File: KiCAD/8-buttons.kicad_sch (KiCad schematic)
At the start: 3 parts, among them U1 74HC165, U2 TLC5916

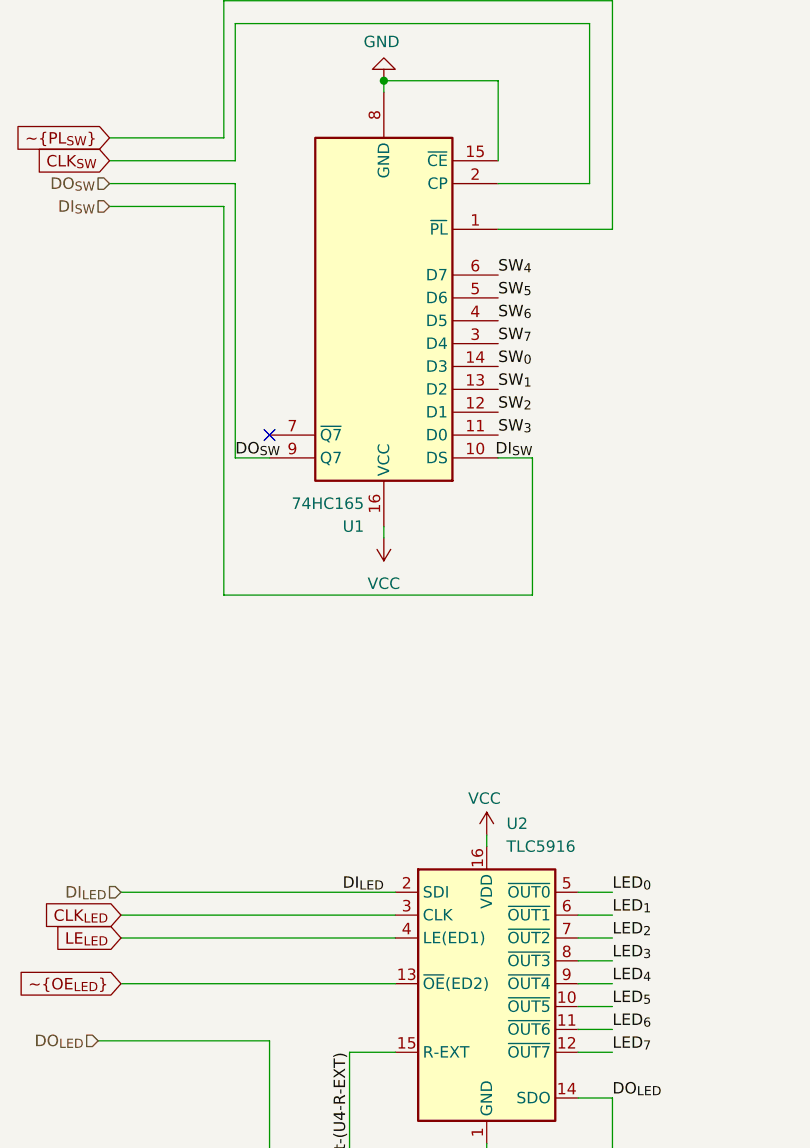
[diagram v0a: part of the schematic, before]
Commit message: Revert "3 rows of 16 buttons; SMT"
This reverts commit c08e4dc0c350e57a2ca7329c2459be699e742724.
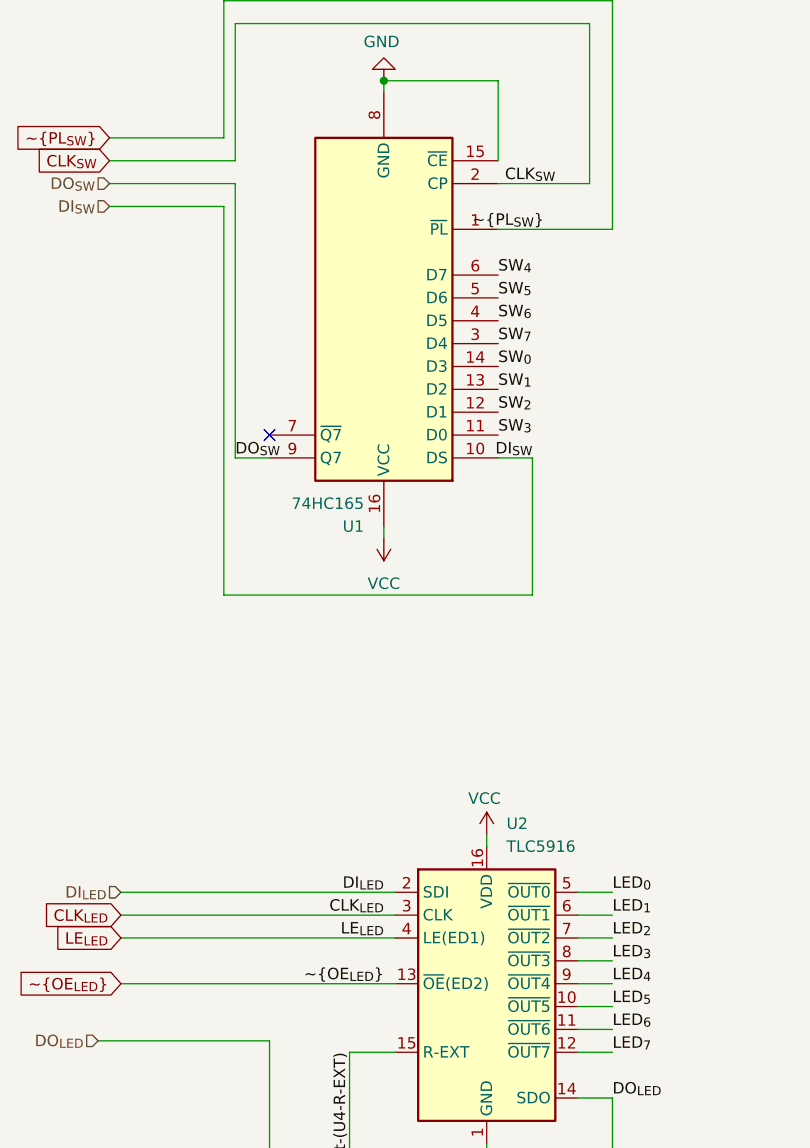
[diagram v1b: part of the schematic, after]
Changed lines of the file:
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@@
+		)
+	)
+	(label "~{OE_{LED}}"
+		(at 58.42 132.08 180)
+		(effects
+			(font
+				(size 1.27 1.27)
+			)
+			(justify right bottom)
 		)
 	)
@@
 		)
 	)
+	(label "LE_{LED}"
+		(at 58.42 127 180)
+		(effects
+			(font
+				(size 1.27 1.27)
+			)
+			(justify right bottom)
+		)
+	)
 	(label "LED_{1}"
 		(at 151.13 83.82 180)
@@
 		)
 	)
+	(label "CLK_{SW}"
+		(at 77.47 43.18 180)
+		(effects
+			(font
+				(size 1.27 1.27)
+			)
+			(justify right bottom)
+		)
+	)
+	(label "CLK_{LED}"
+		(at 58.42 124.46 180)
+		(effects
+			(font
+				(size 1.27 1.27)
+			)
+			(justify right bottom)
+		)
+	)
 	(label "SW_{0}"
 		(at 123.19 78.74 180)
@@
 		(effects
 			(font
+				(size 1.27 1.27)
+			)
+			(justify right bottom)
+		)
+	)
+	(label "~{PL_{SW}}"
+		(at 76.2 48.26 180)
+		(effects
+			(font

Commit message: 3 rows of 16 buttons; SMT
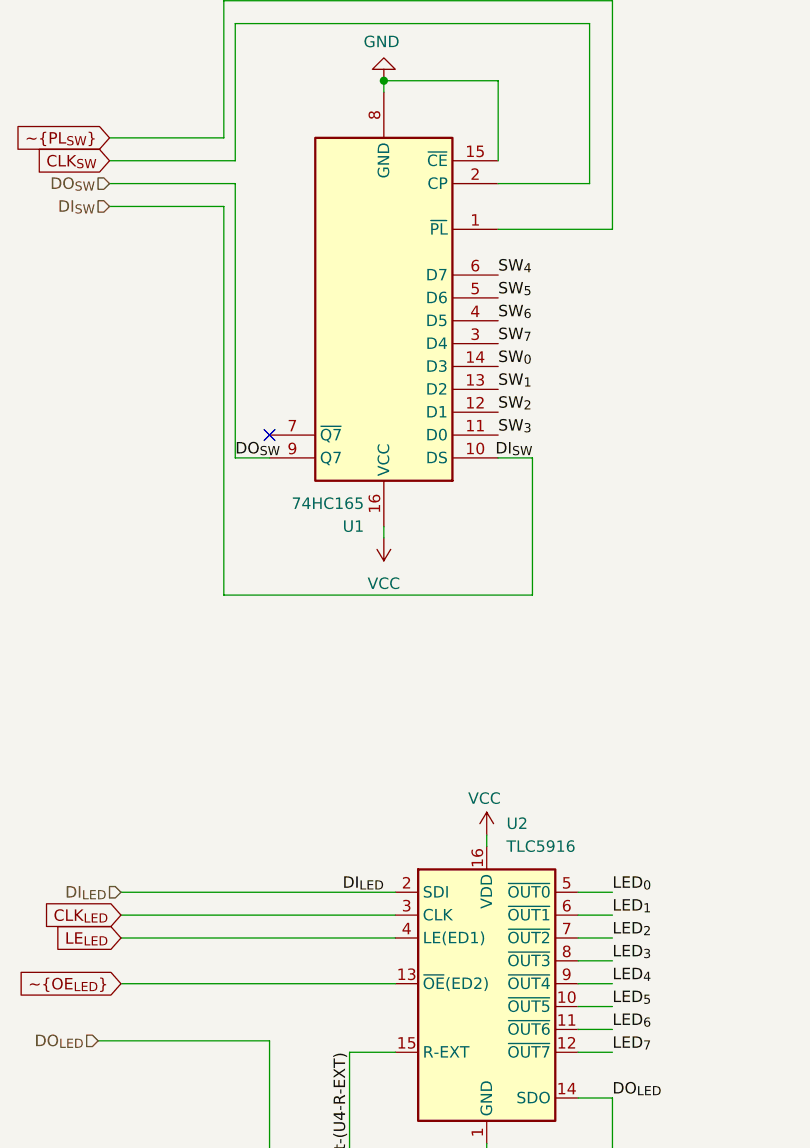
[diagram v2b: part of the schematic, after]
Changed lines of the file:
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@@
-		)
-	)
-	(label "~{OE_{LED}}"
-		(at 58.42 132.08 180)
-		(effects
-			(font
-				(size 1.27 1.27)
-			)
-			(justify right bottom)
 		)
 	)
@@
 		)
 	)
-	(label "LE_{LED}"
-		(at 58.42 127 180)
-		(effects
-			(font
-				(size 1.27 1.27)
-			)
-			(justify right bottom)
-		)
-	)
 	(label "LED_{1}"
 		(at 151.13 83.82 180)
@@
 		)
 	)
-	(label "CLK_{SW}"
-		(at 77.47 43.18 180)
-		(effects
-			(font
-				(size 1.27 1.27)
-			)
-			(justify right bottom)
-		)
-	)
-	(label "CLK_{LED}"
-		(at 58.42 124.46 180)
-		(effects
-			(font
-				(size 1.27 1.27)
-			)
-			(justify right bottom)
-		)
-	)
 	(label "SW_{0}"
 		(at 123.19 78.74 180)
@@
 		(effects
 			(font
-				(size 1.27 1.27)
-			)
-			(justify right bottom)
-		)
-	)
-	(label "~{PL_{SW}}"
-		(at 76.2 48.26 180)
-		(effects
-			(font
